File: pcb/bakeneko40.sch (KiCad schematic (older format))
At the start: 116 parts, among them J1 JST SH 4-pin, J2 AVR-ISP-6, SW1 SW_Push, U1 ATmega32U2-MU, U2 SRV05-4, Y1 16MHz

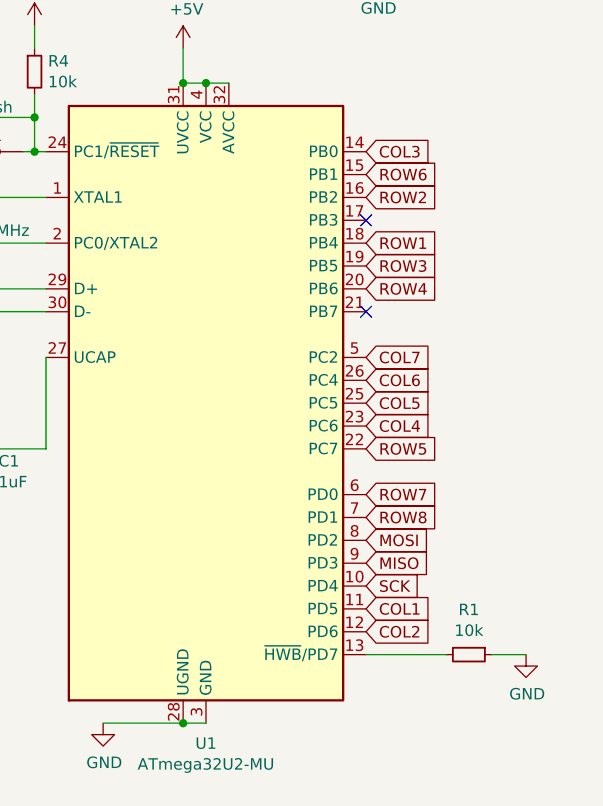
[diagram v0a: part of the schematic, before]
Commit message: final pcb and case
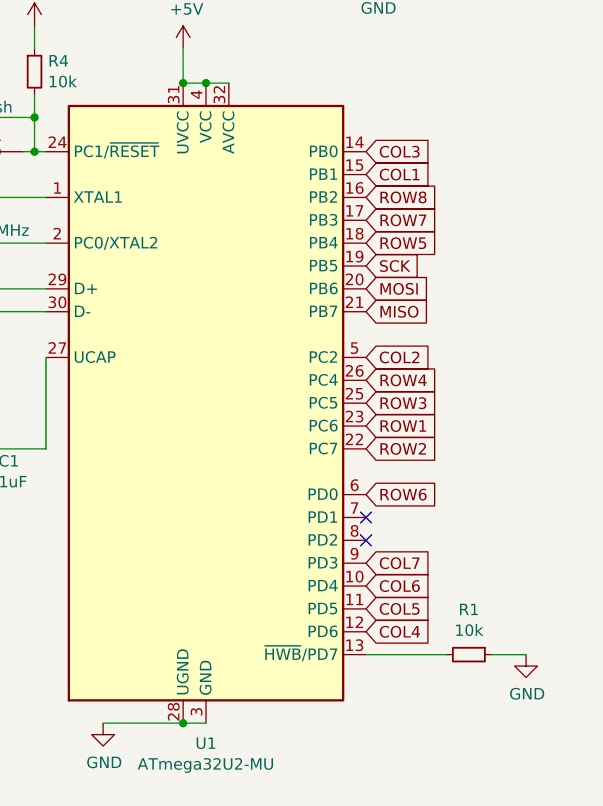
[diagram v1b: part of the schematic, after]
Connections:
- net COL1: now also U1.15 (PB1); no longer U1.11 (PD5)
- net COL2: now also U1.5 (PC2); no longer U1.12 (PD6)
- net COL4: now also U1.12 (PD6); no longer U1.23 (PC6)
- net COL5: now also U1.11 (PD5); no longer U1.25 (PC5)
- net COL6: now also U1.10 (PD4); no longer U1.26 (PC4)
- net COL7: now also U1.9 (PD3); no longer U1.5 (PC2)
- net MISO: now also U1.21 (PB7); no longer U1.9 (PD3)
- net MOSI: now also U1.20 (PB6); no longer U1.8 (PD2)
- net ROW1: now also U1.23 (PC6); no longer U1.18 (PB4)
- net ROW2: now also U1.22 (PC7); no longer U1.16 (PB2)
- net ROW3: now also U1.25 (PC5); no longer U1.19 (PB5)
- net ROW4: now also U1.26 (PC4); no longer U1.20 (PB6)
- net ROW5: now also U1.18 (PB4); no longer U1.22 (PC7)
- net ROW6: now also U1.6 (PD0); no longer U1.15 (PB1)
- net ROW7: now also U1.17 (PB3); no longer U1.6 (PD0)
- net ROW8: now also U1.16 (PB2); no longer U1.7 (PD1)
- net SCK: now also U1.19 (PB5); no longer U1.10 (PD4)
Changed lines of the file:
@@
 Text GLabel 7200 1200 2    50   Input ~ 0
 SCK
-Text GLabel 10200 3750 2    50   Input ~ 0
-MOSI
 $Comp
 L Power_Protection:SRV05-4 U2
@@
 Text GLabel 7800 3850 1    50   Input ~ 0
 COL7
+Text GLabel 10200 3150 2    50   Input ~ 0
+ROW3
+Text GLabel 10200 3050 2    50   Input ~ 0
+ROW4
 Text GLabel 10200 2450 2    50   Input ~ 0
-ROW1
+ROW5
+Text GLabel 10200 2350 2    50   Input ~ 0
+ROW7
 Text GLabel 10200 2250 2    50   Input ~ 0
-ROW2
-Text GLabel 10200 2550 2    50   Input ~ 0
-ROW3
-Text GLabel 10200 2650 2    50   Input ~ 0
-ROW4
-Text GLabel 10200 3350 2    50   Input ~ 0
-ROW5
+ROW8
 Text GLabel 10200 2150 2    50   Input ~ 0
-ROW6
-Text GLabel 10200 3550 2    50   Input ~ 0
-ROW7
-Text GLabel 10200 3650 2    50   Input ~ 0
-ROW8
-Text GLabel 10200 4050 2    50   Input ~ 0
 COL1
-Text GLabel 10200 4150 2    50   Input ~ 0
+Text GLabel 10200 2950 2    50   Input ~ 0
 COL2
 Text GLabel 10200 2050 2    50   Input ~ 0
 COL3
-Text GLabel 10200 3250 2    50   Input ~ 0
+Text GLabel 10200 4150 2    50   Input ~ 0
 COL4
-Text GLabel 10200 3150 2    50   Input ~ 0
+Text GLabel 10200 4050 2    50   Input ~ 0
 COL5
-Text GLabel 10200 3050 2    50   Input ~ 0
+Text GLabel 10200 3950 2    50   Input ~ 0
 COL6
-Text GLabel 10200 2950 2    50   Input ~ 0
+Text GLabel 10200 3850 2    50   Input ~ 0
 COL7
 Connection ~ 1800 6050
@@
 Wire Wire Line
 	10200 4250 10550 4250
-Text GLabel 10200 3850 2    50   Input ~ 0
+Text GLabel 10200 2750 2    50   Input ~ 0
 MISO
 Wire Wire Line
 	9400 1750 9400 1600
-Text GLabel 10200 3950 2    50   Input ~ 0
+Text GLabel 10200 2550 2    50   Input ~ 0
 SCK
 Wire Wire Line
@@
 Wire Wire Line
 	8750 1900 8750 2050
-NoConn ~ 10200 2350
-NoConn ~ 10200 2750
 Wire Wire Line
 	9400 1750 9500 1750
@@
 	1    0    0    -1
 $EndComp
+Text GLabel 10200 3250 2    50   Input ~ 0
+ROW1
+Text GLabel 10200 2650 2    50   Input ~ 0
+MOSI
+NoConn ~ 10200 3650
+Text GLabel 10200 3550 2    50   Input ~ 0
+ROW6
+Text GLabel 10200 3350 2    50   Input ~ 0
+ROW2
+NoConn ~ 10200 3750
 $EndSCHEMATC
